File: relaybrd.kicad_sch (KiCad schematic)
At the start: 1 part, among them J7 5499922-4

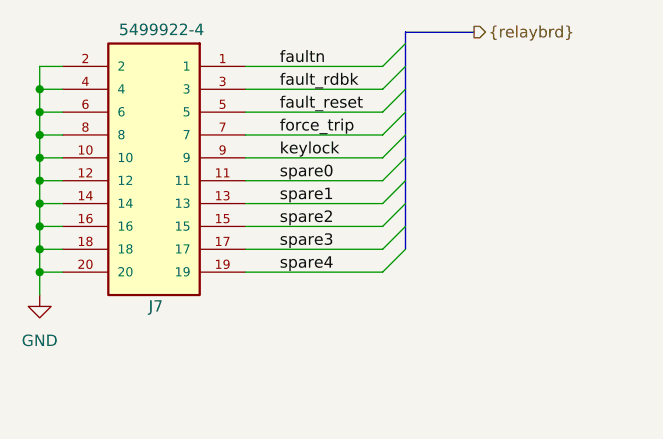
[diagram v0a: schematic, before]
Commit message: push from windows
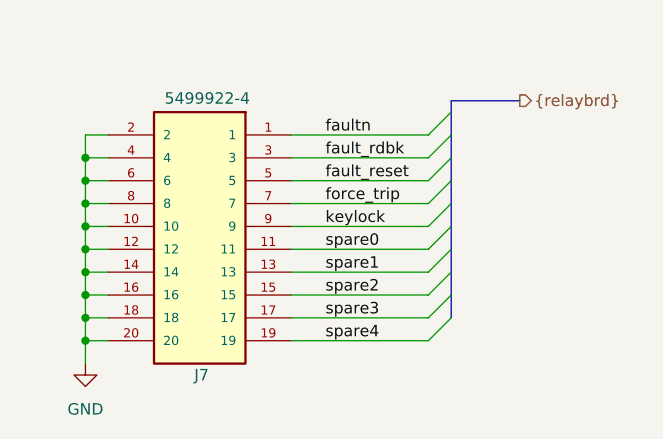
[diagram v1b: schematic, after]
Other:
- moved on the sheet: J7
